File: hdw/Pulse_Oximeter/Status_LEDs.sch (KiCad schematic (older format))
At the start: 30 parts

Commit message: Continued schematic development
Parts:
- added C?: 0.1uF, Capacitors_SMD:C_0402, symbol Custom_Library:C_Custom
- added D?: Red, LEDs:LED_0402, symbol Device:LED
- added R?: 1k, Resistors_SMD:R_0402, symbol Custom_Library:R_Custom
- added R?: 10k, Resistors_SMD:R_0402, symbol Custom_Library:R_Custom
- added U?: 74LVC1G97, Package_TO_SOT_SMD:SOT-363_SC-70-6, symbol Custom_Library:74LVC1G97_Power_NOT
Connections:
- net labels added: I2C_Error_LED
- net labels removed: ETH_Error_LED
- wire segments 30 -> 35
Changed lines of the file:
@@
 $Descr A 11000 8500
 encoding utf-8
-Sheet 14 19
+Sheet 19 19
 Title ""
 Date ""
@@
 Wire Wire Line
 	7850 2220 7850 2300
-Text GLabel 7770 2220 0    50   Input ~ 0
-ETH_Error_LED
 Wire Wire Line
 	7770 2220 7850 2220
@@
 Text GLabel 3770 4220 0    50   Input ~ 0
 CPU_Exception_LED
+Text GLabel 7770 2220 0    50   Input ~ 0
+I2C_Error_LED
+$Comp
+L Custom_Library:C_Custom C?
+U 1 1 5EB97A5A
+P 2290 3530
+AR Path="/5BAAE1F3/5EB97A5A" Ref="C?"  Part="1"
+AR Path="/5BAAE1CB/5EB97A5A" Ref="C?"  Part="1"
+AR Path="/5BE48F98/5EB97A5A" Ref="C?"  Part="1"
+AR Path="/5CAD2D97/5EB97A5A" Ref="C?"  Part="1"
+AR Path="/5CB7A8BC/5EB97A5A" Ref="C?"  Part="1"
+AR Path="/5E6AF016/5EB97A5A" Ref="C?"  Part="1"
+AR Path="/5EAE4AE4/5EB97A5A" Ref="C?"  Part="1"
+F 0 "C?" H 2315 3630 50  0000 L CNN
+F 1 "0.1uF" H 2315 3430 50  0000 L CNN
+F 2 "Capacitors_SMD:C_0402" H 2328 3380 50  0001 C CNN
+F 3 "" H 2315 3630 50  0001 C CNN
+F 4 "490-10701-1-ND" H 2715 4030 60  0001 C CNN "Digi-Key PN"
+F 5 "0402" H 2140 3630 50  0000 R CNN "display_footprint"
+F 6 "50V" H 2140 3530 50  0000 R CNN "Voltage"
+F 7 "X7R" H 2140 3430 50  0000 R CNN "Dielectric"
+	1    2290 3530
+	-1   0    0    -1
+$EndComp
+Wire Wire Line
+	2650 4220 2970 4220
+Wire Wire Line
+	2970 4220 2970 4100
+$Comp
+L Custom_Library:R_Custom R?
+U 1 1 5EB97A6A
+P 2970 3650
+AR Path="/5BAAE1F3/5EB97A6A" Ref="R?"  Part="1"
+AR Path="/5BAAE1DC/5EB97A6A" Ref="R?"  Part="1"
+AR Path="/5BAAE16C/5EB97A6A" Ref="R?"  Part="1"
+AR Path="/5BB844FD/5EB97A6A" Ref="R?"  Part="1"
+AR Path="/5BF346B3/5EB97A6A" Ref="R?"  Part="1"
+AR Path="/5CAD2D97/5EB97A6A" Ref="R?"  Part="1"
+AR Path="/5CB7A8BC/5EB97A6A" Ref="R?"  Part="1"
+AR Path="/5E6AF016/5EB97A6A" Ref="R?"  Part="1"
+AR Path="/5EAE4AE4/5EB97A6A" Ref="R?"  Part="1"
+F 0 "R?" H 2910 3650 50  0000 R CNN
+F 1 "1k" V 2970 3650 50  0000 C CNN
+F 2 "Resistors_SMD:R_0402" H 2970 3650 50  0001 C CNN
+F 3 "" H 2970 3650 50  0001 C CNN
+F 4 "0402" H 3040 3730 50  0000 L CNN "display_footprint"
+F 5 "1%" H 3040 3650 50  0000 L CNN "Tolerance"
+F 6 "1/16W" H 3040 3580 50  0000 L CNN "Wattage"
+F 7 "541-1.00KLCT-ND" H 3270 4050 60  0001 C CNN "Digi-Key PN"
+	1    2970 3650
+	-1   0    0    -1
+$EndComp
+$Comp
+L power:+3.3V #PWR?
+U 1 1 5EB97A74
+P 2970 3500
+F 0 "#PWR?" H 2970 3350 50  0001 C CNN
+F 1 "+3.3V" H 2970 3640 50  0000 C CNN
+F 2 "" H 2970 3500 50  0001 C CNN
+F 3 "" H 2970 3500 50  0001 C CNN
+	1    2970 3500
+	1    0    0    -1
+$EndComp
+$Comp
+L power:+3.3V #PWR?
+U 1 1 5EB97A7E
+P 2290 3380
+F 0 "#PWR?" H 2290 3230 50  0001 C CNN
+F 1 "+3.3V" H 2290 3520 50  0000 C CNN
+F 2 "" H 2290 3380 50  0001 C CNN
+F 3 "" H 2290 3380 50  0001 C CNN
+	1    2290 3380
+	1    0    0    -1
+$EndComp
+$Comp
+L power:GND #PWR?
+U 1 1 5EB97A88
+P 2290 3680
+F 0 "#PWR?" H 2290 3430 50  0001 C CNN
+F 1 "GND" H 2290 3530 50  0000 C CNN
+F 2 "" H 2290 3680 50  0001 C CNN
+F 3 "" H 2290 3680 50  0001 C CNN
+	1    2290 3680
+	1    0    0    -1
+$EndComp
+$Comp
+L Custom_Library:R_Custom R?
+U 1 1 5EB97A96
+P 1850 4450
+AR Path="/5BAAE1F3/5EB97A96" Ref="R?"  Part="1"
+AR Path="/5BAAE1DC/5EB97A96" Ref="R?"  Part="1"
+AR Path="/5BAAE16C/5EB97A96" Ref="R?"  Part="1"
+AR Path="/5BB844FD/5EB97A96" Ref="R?"  Part="1"
+AR Path="/5BF346B3/5EB97A96" Ref="R?"  Part="1"
+AR Path="/5CAD2D97/5EB97A96" Ref="R?"  Part="1"
+AR Path="/5CB7A8BC/5EB97A96" Ref="R?"  Part="1"
+AR Path="/5E6AF016/5EB97A96" Ref="R?"  Part="1"
+AR Path="/5EAE4AE4/5EB97A96" Ref="R?"  Part="1"
+F 0 "R?" H 1790 4450 50  0000 R CNN
+F 1 "10k" V 1850 4450 50  0000 C CNN
+F 2 "Resistors_SMD:R_0402" H 1850 4450 50  0001 C CNN
+F 3 "" H 1850 4450 50  0001 C CNN
+F 4 "0402" H 1920 4530 50  0000 L CNN "display_footprint"
+F 5 "1%" H 1920 4450 50  0000 L CNN "Tolerance"
+F 6 "1/16W" H 1920 4380 50  0000 L CNN "Wattage"
+F 7 "RMCF0402FT10K0CT-ND" H 1850 4450 50  0001 C CNN "Digi-Key PN"
+	1    1850 4450
+	-1   0    0    -1
+$EndComp
+$Comp
+L power:GND #PWR?
+U 1 1 5EB97AA0
+P 1850 4600
+F 0 "#PWR?" H 1850 4350 50  0001 C CNN
+F 1 "GND" H 1850 4450 50  0000 C CNN
+F 2 "" H 1850 4600 50  0001 C CNN
+F 3 "" H 1850 4600 50  0001 C CNN
+	1    1850 4600
+	1    0    0    -1
+$EndComp
+Wire Wire Line
+	2100 4220 1850 4220
+Wire Wire Line
+	1850 4220 1850 4300
+Wire Wire Line
+	1770 4220 1850 4220
+Connection ~ 1850 4220
+$Comp
+L Device:LED D?
+U 1 1 5EB97AAF
+P 2970 3950
+AR Path="/5BB844FD/5EB97AAF" Ref="D?"  Part="1"
+AR Path="/5BF346B3/5EB97AAF" Ref="D?"  Part="1"
+AR Path="/5BAAE1F3/5EB97AAF" Ref="D?"  Part="1"
+AR Path="/5CAD2D97/5EB97AAF" Ref="D?"  Part="1"
+AR Path="/5CB7A8BC/5EB97AAF" Ref="D?"  Part="1"
+AR Path="/5E6AF016/5EB97AAF" Ref="D?"  Part="1"
+AR Path="/5EAE4AE4/5EB97AAF" Ref="D?"  Part="1"
+F 0 "D?" V 3009 3833 50  0000 R CNN
+F 1 "Red" V 2918 3833 50  0000 R CNN
+F 2 "LEDs:LED_0402" H 2970 3950 50  0001 C CNN
+F 3 "~" H 2970 3950 50  0001 C CNN
+F 4 "1497-1174-1-ND" H 2970 3950 50  0001 C CNN "Digi-Key PN"
+	1    2970 3950
+	0    -1   -1   0
+$EndComp
+$Comp
+L power:+3.3V #PWR?
+U 1 1 5EB97AB9
+P 2400 4120
+F 0 "#PWR?" H 2400 3970 50  0001 C CNN
+F 1 "+3.3V" H 2400 4260 50  0000 C CNN
+F 2 "" H 2400 4120 50  0001 C CNN
+F 3 "" H 2400 4120 50  0001 C CNN
+	1    2400 4120
+	1    0    0    -1
+$EndComp
+$Comp
+L power:GND #PWR?
+U 1 1 5EB97AC3
+P 2400 4320
+F 0 "#PWR?" H 2400 4070 50  0001 C CNN
+F 1 "GND" H 2400 4170 50  0000 C CNN
+F 2 "" H 2400 4320 50  0001 C CNN
+F 3 "" H 2400 4320 50  0001 C CNN
+	1    2400 4320
+	1    0    0    -1
+$EndComp
+$Comp
+L Custom_Library:74LVC1G97_Power_NOT U?
+U 1 1 5EB97ACE
+P 2400 4220
+F 0 "U?" H 2460 4370 50  0000 L CNN
+F 1 "74LVC1G97" H 2460 4070 50  0000 L CNN
+F 2 "Package_TO_SOT_SMD:SOT-363_SC-70-6" H 2450 4220 50  0001 C CNN
+F 3 "http://www.ti.com/lit/ds/symlink/sn74lvc1g97.pdf" H 2450 4220 50  0001 C CNN
+F 4 "296-15582-1-ND" H 2400 4220 50  0001 C CNN "Digi-Key PN"
+	1    2400 4220
+	1    0    0    -1
+$EndComp
 $EndSCHEMATC

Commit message: Added display circuits
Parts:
- removed U? (x7): 74LVC1G97, Package_TO_SOT_SMD:SOT-363_SC-70-6, symbol Custom_Library:74LVC1G97_Power_NOT
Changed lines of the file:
@@
 EESchema Schematic File Version 4
+LIBS:Pulse_Oximeter-cache
 EELAYER 30 0
 EELAYER END
@@
 	1    0    0    -1
 $EndComp
-$Comp
-L Custom_Library:74LVC1G97_Power_NOT U?
-U 1 1 5E499235
-P 2400 2220
-F 0 "U?" H 2460 2370 50  0000 L CNN
-F 1 "74LVC1G97" H 2460 2070 50  0000 L CNN
-F 2 "Package_TO_SOT_SMD:SOT-363_SC-70-6" H 2450 2220 50  0001 C CNN
-F 3 "http://www.ti.com/lit/ds/symlink/sn74lvc1g97.pdf" H 2450 2220 50  0001 C CNN
-F 4 "296-15582-1-ND" H 2400 2220 50  0001 C CNN "Digi-Key PN"
-	1    2400 2220
-	1    0    0    -1
-$EndComp
-$Comp
-L Custom_Library:74LVC1G97_Power_NOT U?
-U 1 1 5E499F9B
-P 4400 2220
-F 0 "U?" H 4460 2370 50  0000 L CNN
-F 1 "74LVC1G97" H 4460 2070 50  0000 L CNN
-F 2 "Package_TO_SOT_SMD:SOT-363_SC-70-6" H 4450 2220 50  0001 C CNN
-F 3 "http://www.ti.com/lit/ds/symlink/sn74lvc1g97.pdf" H 4450 2220 50  0001 C CNN
-F 4 "296-15582-1-ND" H 4400 2220 50  0001 C CNN "Digi-Key PN"
-	1    4400 2220
-	1    0    0    -1
-$EndComp
-$Comp
-L Custom_Library:74LVC1G97_Power_NOT U?
-U 1 1 5E49A9B3
-P 6400 2220
-F 0 "U?" H 6460 2370 50  0000 L CNN
-F 1 "74LVC1G97" H 6460 2070 50  0000 L CNN
-F 2 "Package_TO_SOT_SMD:SOT-363_SC-70-6" H 6450 2220 50  0001 C CNN
-F 3 "http://www.ti.com/lit/ds/symlink/sn74lvc1g97.pdf" H 6450 2220 50  0001 C CNN
-F 4 "296-15582-1-ND" H 6400 2220 50  0001 C CNN "Digi-Key PN"
-	1    6400 2220
-	1    0    0    -1
-$EndComp
-$Comp
-L Custom_Library:74LVC1G97_Power_NOT U?
-U 1 1 5E49B430
-P 8400 2220
-F 0 "U?" H 8460 2370 50  0000 L CNN
-F 1 "74LVC1G97" H 8460 2070 50  0000 L CNN
-F 2 "Package_TO_SOT_SMD:SOT-363_SC-70-6" H 8450 2220 50  0001 C CNN
-F 3 "http://www.ti.com/lit/ds/symlink/sn74lvc1g97.pdf" H 8450 2220 50  0001 C CNN
-F 4 "296-15582-1-ND" H 8400 2220 50  0001 C CNN "Digi-Key PN"
-	1    8400 2220
-	1    0    0    -1
-$EndComp
-$Comp
-L Custom_Library:74LVC1G97_Power_NOT U?
-U 1 1 5E49BF58
-P 6400 4220
-F 0 "U?" H 6460 4370 50  0000 L CNN
-F 1 "74LVC1G97" H 6460 4070 50  0000 L CNN
-F 2 "Package_TO_SOT_SMD:SOT-363_SC-70-6" H 6450 4220 50  0001 C CNN
-F 3 "http://www.ti.com/lit/ds/symlink/sn74lvc1g97.pdf" H 6450 4220 50  0001 C CNN
-F 4 "296-15582-1-ND" H 6400 4220 50  0001 C CNN "Digi-Key PN"
-	1    6400 4220
-	1    0    0    -1
-$EndComp
-$Comp
-L Custom_Library:74LVC1G97_Power_NOT U?
-U 1 1 5E49CDEC
-P 4400 4220
-F 0 "U?" H 4460 4370 50  0000 L CNN
-F 1 "74LVC1G97" H 4460 4070 50  0000 L CNN
-F 2 "Package_TO_SOT_SMD:SOT-363_SC-70-6" H 4450 4220 50  0001 C CNN
-F 3 "http://www.ti.com/lit/ds/symlink/sn74lvc1g97.pdf" H 4450 4220 50  0001 C CNN
-F 4 "296-15582-1-ND" H 4400 4220 50  0001 C CNN "Digi-Key PN"
-	1    4400 4220
-	1    0    0    -1
-$EndComp
 Text GLabel 3770 4220 0    50   Input ~ 0
 CPU_Exception_LED
@@
 	1    0    0    -1
 $EndComp
-$Comp
-L Custom_Library:74LVC1G97_Power_NOT U?
-U 1 1 5EB97ACE
-P 2400 4220
-F 0 "U?" H 2460 4370 50  0000 L CNN
-F 1 "74LVC1G97" H 2460 4070 50  0000 L CNN
-F 2 "Package_TO_SOT_SMD:SOT-363_SC-70-6" H 2450 4220 50  0001 C CNN
-F 3 "http://www.ti.com/lit/ds/symlink/sn74lvc1g97.pdf" H 2450 4220 50  0001 C CNN
-F 4 "296-15582-1-ND" H 2400 4220 50  0001 C CNN "Digi-Key PN"
-	1    2400 4220
-	1    0    0    -1
-$EndComp

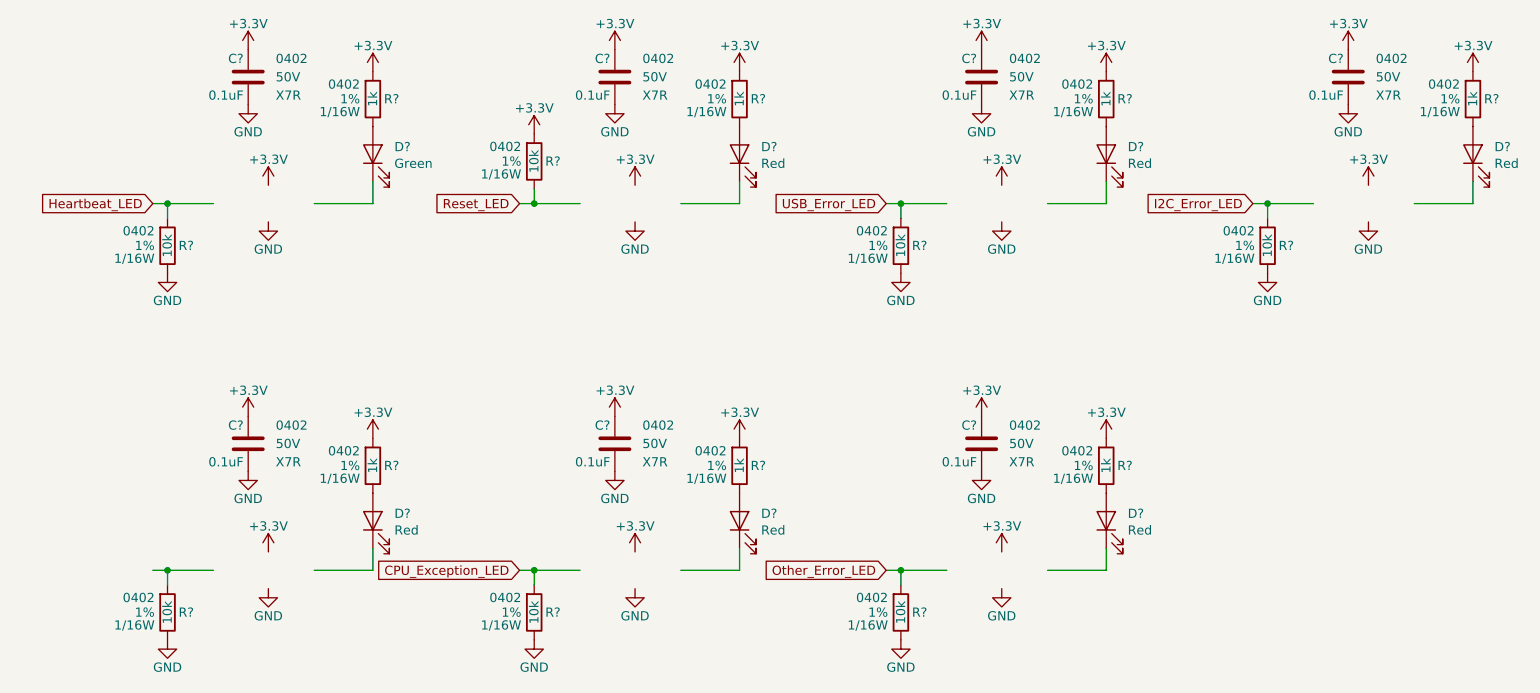
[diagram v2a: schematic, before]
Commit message: few sch additions
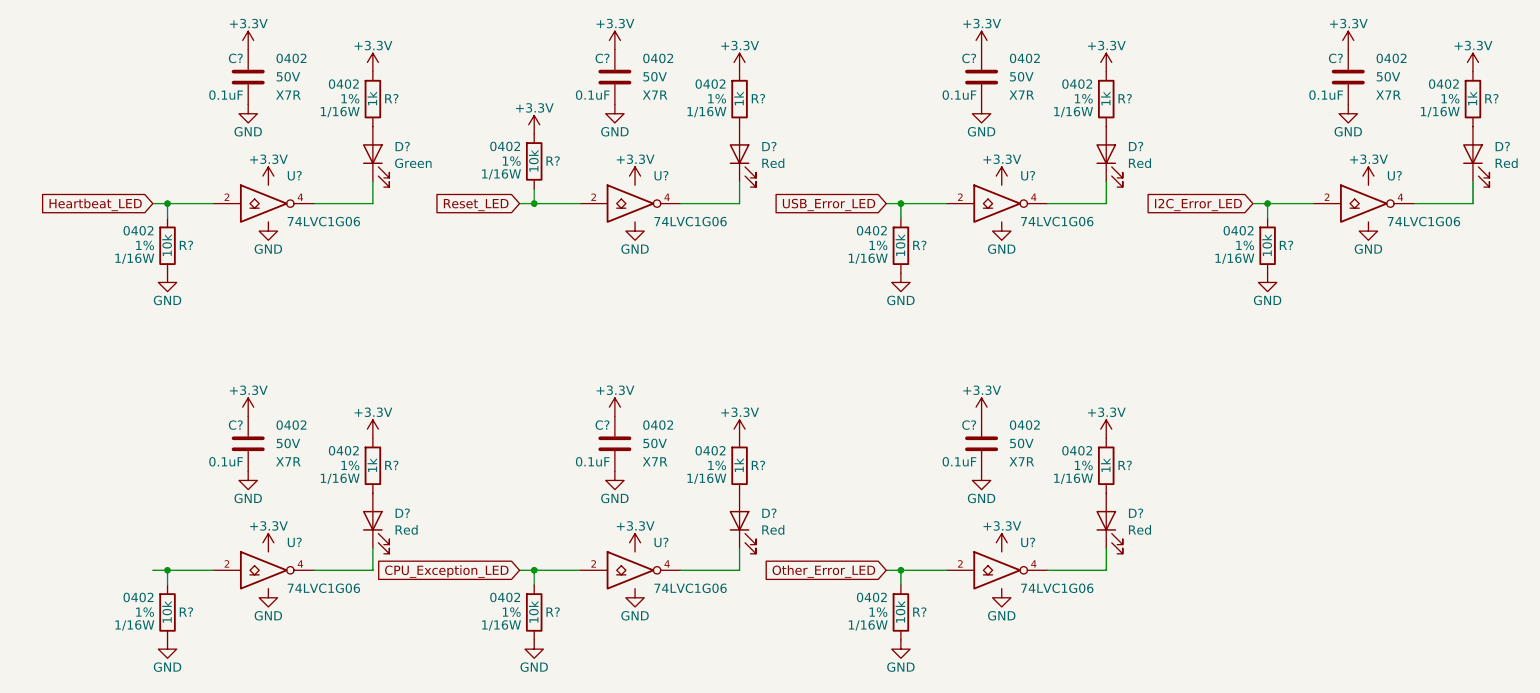
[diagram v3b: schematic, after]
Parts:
- added U? (x7): 74LVC1G06, TO_SOT_Packages_SMD:SOT-353_SC-70-5, symbol Custom_Library:74LVC1G06_Power
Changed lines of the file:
@@
+	1    0    0    -1
+$EndComp
+$Comp
+L Custom_Library:74LVC1G06_Power U?
+U 1 1 5EBB3661
+P 2400 2220
+AR Path="/5EAE4ADE/5EBB3661" Ref="U?"  Part="1"
+AR Path="/5EAE4AE4/5EBB3661" Ref="U?"  Part="1"
+F 0 "U?" H 2500 2370 50  0000 L CNN
+F 1 "74LVC1G06" H 2500 2120 50  0000 L CNN
+F 2 "TO_SOT_Packages_SMD:SOT-353_SC-70-5" H 2400 2270 50  0001 C CNN
+F 3 "http://www.ti.com/lit/ds/symlink/sn74lvc1g06.pdf" H 2400 2220 50  0001 C CNN
+F 4 "296-8484-1-ND" H 2400 2220 50  0001 C CNN "Digi-Key PN"
+	1    2400 2220
+	1    0    0    -1
+$EndComp
+$Comp
+L Custom_Library:74LVC1G06_Power U?
+U 1 1 5EBB3BCA
+P 4400 2220
+AR Path="/5EAE4ADE/5EBB3BCA" Ref="U?"  Part="1"
+AR Path="/5EAE4AE4/5EBB3BCA" Ref="U?"  Part="1"
+F 0 "U?" H 4500 2370 50  0000 L CNN
+F 1 "74LVC1G06" H 4500 2120 50  0000 L CNN
+F 2 "TO_SOT_Packages_SMD:SOT-353_SC-70-5" H 4400 2270 50  0001 C CNN
+F 3 "http://www.ti.com/lit/ds/symlink/sn74lvc1g06.pdf" H 4400 2220 50  0001 C CNN
+F 4 "296-8484-1-ND" H 4400 2220 50  0001 C CNN "Digi-Key PN"
+	1    4400 2220
+	1    0    0    -1
+$EndComp
+$Comp
+L Custom_Library:74LVC1G06_Power U?
+U 1 1 5EBB465B
+P 6400 2220
+AR Path="/5EAE4ADE/5EBB465B" Ref="U?"  Part="1"
+AR Path="/5EAE4AE4/5EBB465B" Ref="U?"  Part="1"
+F 0 "U?" H 6500 2370 50  0000 L CNN
+F 1 "74LVC1G06" H 6500 2120 50  0000 L CNN
+F 2 "TO_SOT_Packages_SMD:SOT-353_SC-70-5" H 6400 2270 50  0001 C CNN
+F 3 "http://www.ti.com/lit/ds/symlink/sn74lvc1g06.pdf" H 6400 2220 50  0001 C CNN
+F 4 "296-8484-1-ND" H 6400 2220 50  0001 C CNN "Digi-Key PN"
+	1    6400 2220
+	1    0    0    -1
+$EndComp
+$Comp
+L Custom_Library:74LVC1G06_Power U?
+U 1 1 5EBB4E70
+P 8400 2220
+AR Path="/5EAE4ADE/5EBB4E70" Ref="U?"  Part="1"
+AR Path="/5EAE4AE4/5EBB4E70" Ref="U?"  Part="1"
+F 0 "U?" H 8500 2370 50  0000 L CNN
+F 1 "74LVC1G06" H 8500 2120 50  0000 L CNN
+F 2 "TO_SOT_Packages_SMD:SOT-353_SC-70-5" H 8400 2270 50  0001 C CNN
+F 3 "http://www.ti.com/lit/ds/symlink/sn74lvc1g06.pdf" H 8400 2220 50  0001 C CNN
+F 4 "296-8484-1-ND" H 8400 2220 50  0001 C CNN "Digi-Key PN"
+	1    8400 2220
+	1    0    0    -1
+$EndComp
+$Comp
+L Custom_Library:74LVC1G06_Power U?
+U 1 1 5EBB56C7
+P 4400 4220
+AR Path="/5EAE4ADE/5EBB56C7" Ref="U?"  Part="1"
+AR Path="/5EAE4AE4/5EBB56C7" Ref="U?"  Part="1"
+F 0 "U?" H 4500 4370 50  0000 L CNN
+F 1 "74LVC1G06" H 4500 4120 50  0000 L CNN
+F 2 "TO_SOT_Packages_SMD:SOT-353_SC-70-5" H 4400 4270 50  0001 C CNN
+F 3 "http://www.ti.com/lit/ds/symlink/sn74lvc1g06.pdf" H 4400 4220 50  0001 C CNN
+F 4 "296-8484-1-ND" H 4400 4220 50  0001 C CNN "Digi-Key PN"
+	1    4400 4220
+	1    0    0    -1
+$EndComp
+$Comp
+L Custom_Library:74LVC1G06_Power U?
+U 1 1 5EBB64EE
+P 6400 4220
+AR Path="/5EAE4ADE/5EBB64EE" Ref="U?"  Part="1"
+AR Path="/5EAE4AE4/5EBB64EE" Ref="U?"  Part="1"
+F 0 "U?" H 6500 4370 50  0000 L CNN
+F 1 "74LVC1G06" H 6500 4120 50  0000 L CNN
+F 2 "TO_SOT_Packages_SMD:SOT-353_SC-70-5" H 6400 4270 50  0001 C CNN
+F 3 "http://www.ti.com/lit/ds/symlink/sn74lvc1g06.pdf" H 6400 4220 50  0001 C CNN
+F 4 "296-8484-1-ND" H 6400 4220 50  0001 C CNN "Digi-Key PN"
+	1    6400 4220
+	1    0    0    -1
+$EndComp
+$Comp
+L Custom_Library:74LVC1G06_Power U?
+U 1 1 5EBB6CE5
+P 2400 4220
+AR Path="/5EAE4ADE/5EBB6CE5" Ref="U?"  Part="1"
+AR Path="/5EAE4AE4/5EBB6CE5" Ref="U?"  Part="1"
+F 0 "U?" H 2500 4370 50  0000 L CNN
+F 1 "74LVC1G06" H 2500 4120 50  0000 L CNN
+F 2 "TO_SOT_Packages_SMD:SOT-353_SC-70-5" H 2400 4270 50  0001 C CNN
+F 3 "http://www.ti.com/lit/ds/symlink/sn74lvc1g06.pdf" H 2400 4220 50  0001 C CNN
+F 4 "296-8484-1-ND" H 2400 4220 50  0001 C CNN "Digi-Key PN"
+	1    2400 4220
 	1    0    0    -1
 $EndComp

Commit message: More sch work
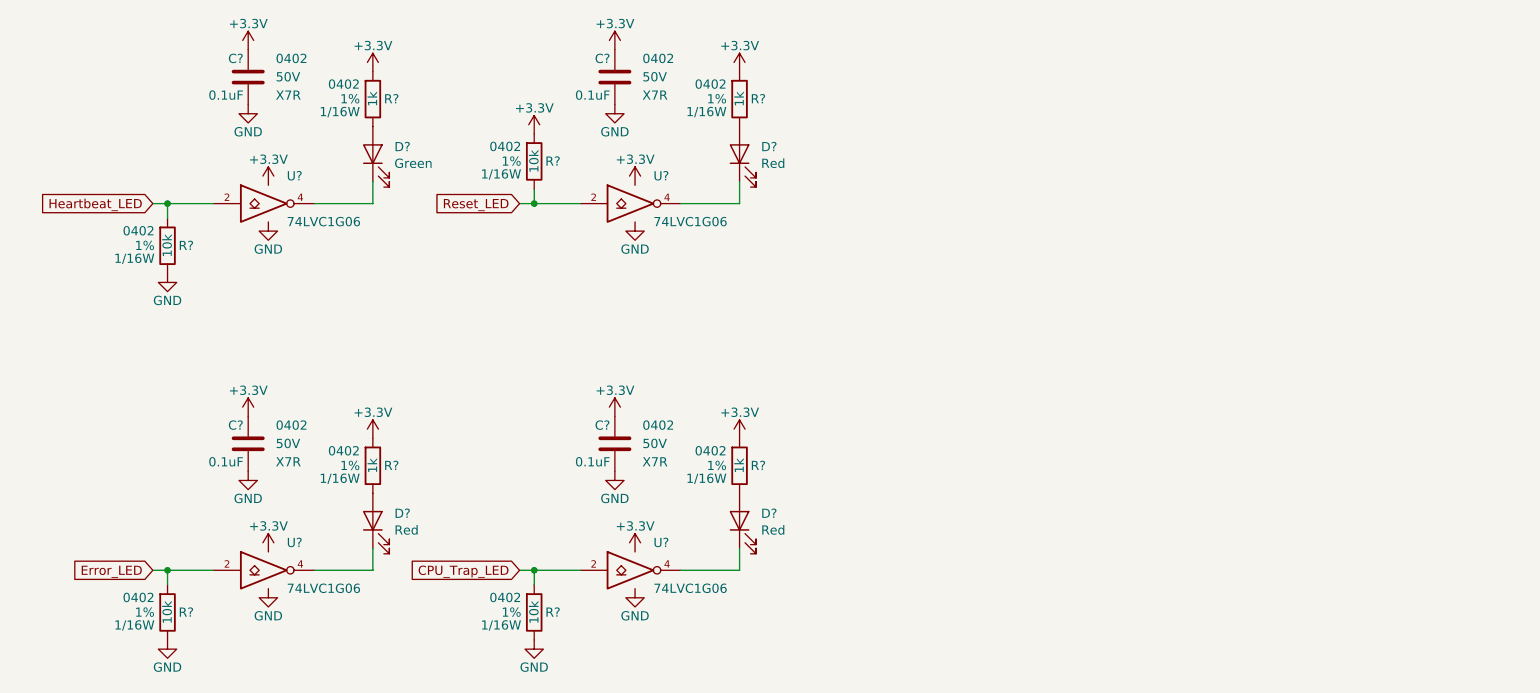
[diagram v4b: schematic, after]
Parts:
- removed C? (x3): 0.1uF, Capacitors_SMD:C_0402, symbol Custom_Library:C_Custom
- removed D? (x3): Red, LEDs:LED_0402, symbol Device:LED
- removed R? (x3): 1k, Resistors_SMD:R_0402, symbol Custom_Library:R_Custom
- removed R? (x3): 10k, Resistors_SMD:R_0402, symbol Custom_Library:R_Custom
- removed U? (x3): 74LVC1G06, TO_SOT_Packages_SMD:SOT-353_SC-70-5, symbol Custom_Library:74LVC1G06_Power
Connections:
- net labels added: CPU_Trap_LED, Error_LED
- net labels removed: CPU_Exception_LED, I2C_Error_LED, Other_Error_LED, USB_Error_LED
- wire segments 35 -> 20
